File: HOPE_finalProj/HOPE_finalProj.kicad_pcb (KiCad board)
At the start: 2 copper layers, 69.3 x 95 mm, 39 parts, among them M1 Mixer, SW1 SW_Push_DPDT, SW2 SW_SPDT, U1 LM386N-3_NOPB, U2 NE5534, U3 NE5534, U4 LM386N-3_NOPB, Y1 Crystal

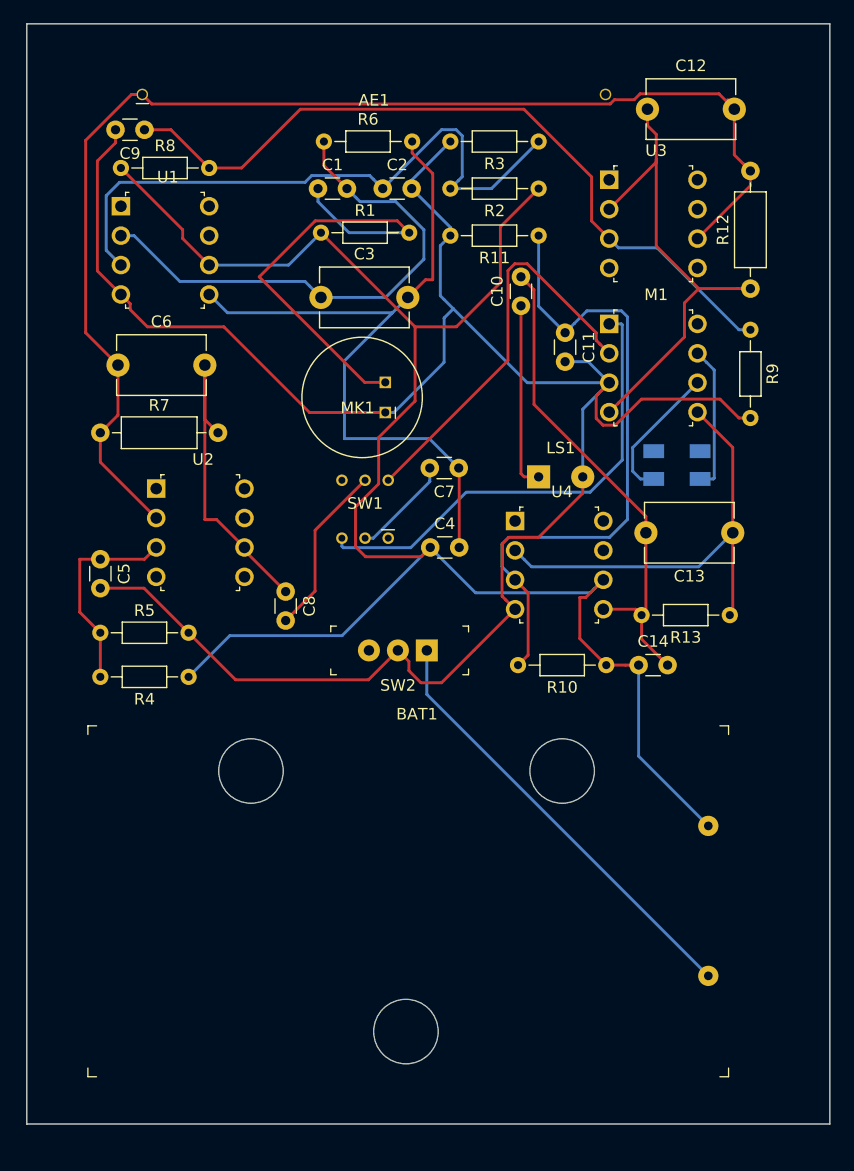
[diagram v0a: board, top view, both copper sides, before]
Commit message: Doing layout
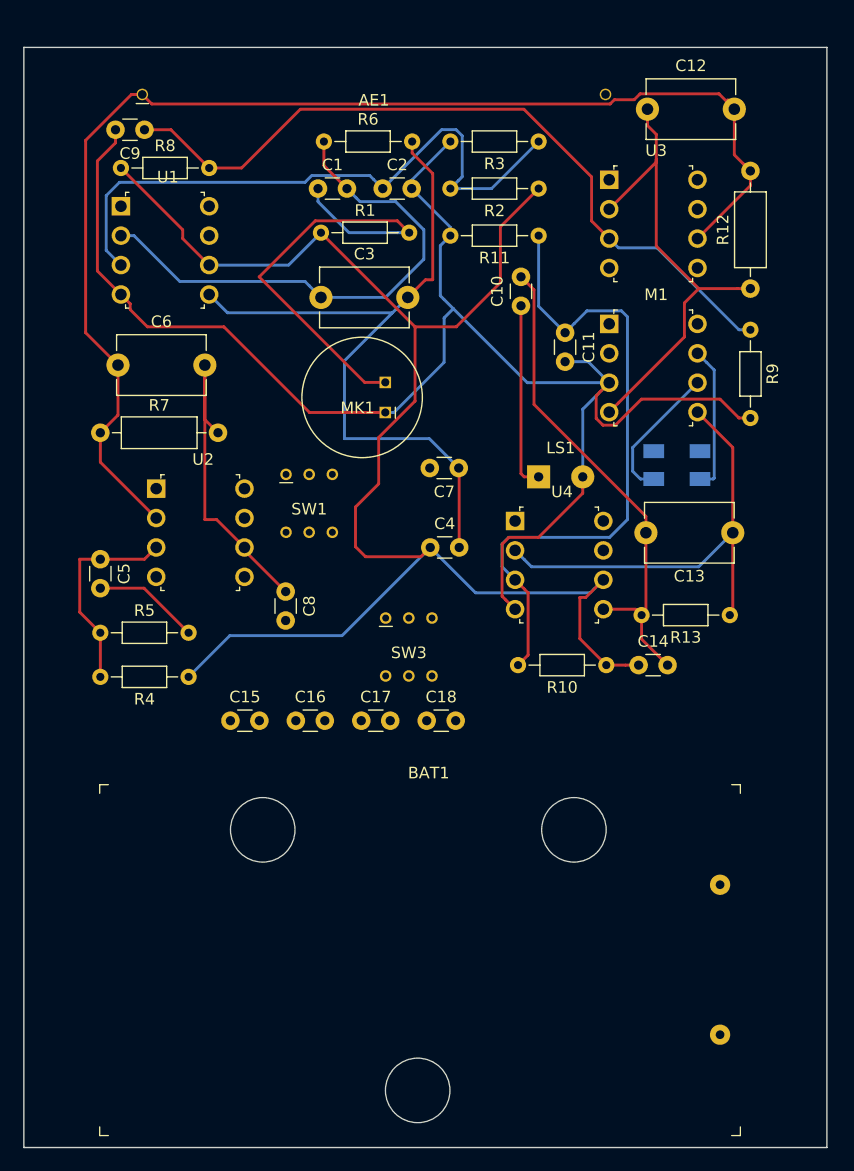
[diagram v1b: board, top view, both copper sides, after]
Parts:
- removed SW2: SW_SPDT, digikey-footprints:Switch_Slide_11.6x4mm_EG1218
- added C15: 1u, Capacitor_THT:C_Disc_D3.0mm_W1.6mm_P2.50mm, F.Cu at (121.2, 114.5)
- added C16: 1u, Capacitor_THT:C_Disc_D3.0mm_W1.6mm_P2.50mm, F.Cu at (126.9, 114.5)
- added C17: 1u, Capacitor_THT:C_Disc_D3.0mm_W1.6mm_P2.50mm, F.Cu at (132.5, 114.5)
- added C18: 1u, Capacitor_THT:C_Disc_D3.0mm_W1.6mm_P2.50mm, F.Cu at (138.2, 114.5)
- added SW3: SW_Push_DPDT, HOPE_finalProj_lib:DPDT_Switch, F.Cu at (136.6, 108.2)
- moved BAT1 5.18 mm to (150.9, 124.0)
- moved SW1 4.85 mm to (128.0, 95.8), turned to 0 degrees
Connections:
- BAT1 pad NEG: Net-(BAT1-PadNEG) -> GND
- C14 pad 1: VCC -> speaker_VCC
- M1 pad 8: (no net) -> VCC
- SW1 pad 1: (no net) -> Net-(C15-Pad1)
- SW1 pad 2: Net-(C7-Pad2) -> Net-(M1-Pad1)
- SW1 pad 3: Net-(M1-Pad1) -> Net-(C7-Pad2)
- SW1 pad 4: Net-(M1-Pad2) -> Net-(C8-Pad2)
- SW1 pad 5: Net-(C8-Pad2) -> Net-(M1-Pad2)
- SW1 pad 6: (no net) -> Net-(C16-Pad2)
- U1 pad 1: (no net) -> Net-(U1-Pad1)
- U1 pad 7: (no net) -> Net-(U1-Pad7)
- U1 pad 8: (no net) -> Net-(U1-Pad8)
- U2 pad 1: (no net) -> Net-(U2-Pad1)
- U2 pad 4: (no net) -> GND
- U2 pad 5: (no net) -> Net-(U2-Pad5)
- U2 pad 7: (no net) -> VCC
- U2 pad 8: (no net) -> Net-(U2-Pad8)
- U3 pad 1: (no net) -> Net-(U3-Pad1)
- U3 pad 4: (no net) -> GND
- U3 pad 5: (no net) -> Net-(U3-Pad5)
- U3 pad 7: (no net) -> transmitter_VCC
- U3 pad 8: (no net) -> Net-(U3-Pad8)
- U4 pad 1: (no net) -> Net-(U4-Pad1)
- U4 pad 6: VCC -> speaker_VCC
- U4 pad 7: (no net) -> Net-(U4-Pad7)
- U4 pad 8: (no net) -> Net-(U4-Pad8)
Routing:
- net Net-(M1-Pad1): track 40.9 -> 0.00 mm
- net Net-(BAT1-PadNEG): track 38.2 -> 0.00 mm
- net GND: track 182.1 -> 146.9 mm
- net Net-(M1-Pad2): track 35.0 -> 0.00 mm
- net VCC: track 151.7 -> 135.3 mm
- net Net-(C8-Pad2): track 15.0 -> 0.00 mm
- net Net-(C7-Pad2): track 8.78 -> 0.00 mm
